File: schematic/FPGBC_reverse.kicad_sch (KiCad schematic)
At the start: 7 parts, among them IC1 CH32V203C8T6, J1 Conn_01x06_Pin, U1 GW2AR-LV18EQ144PC8_17, U2 24C04C, U3 W25Q128JVS, U4 EA3058QD, U5 TCD8002D

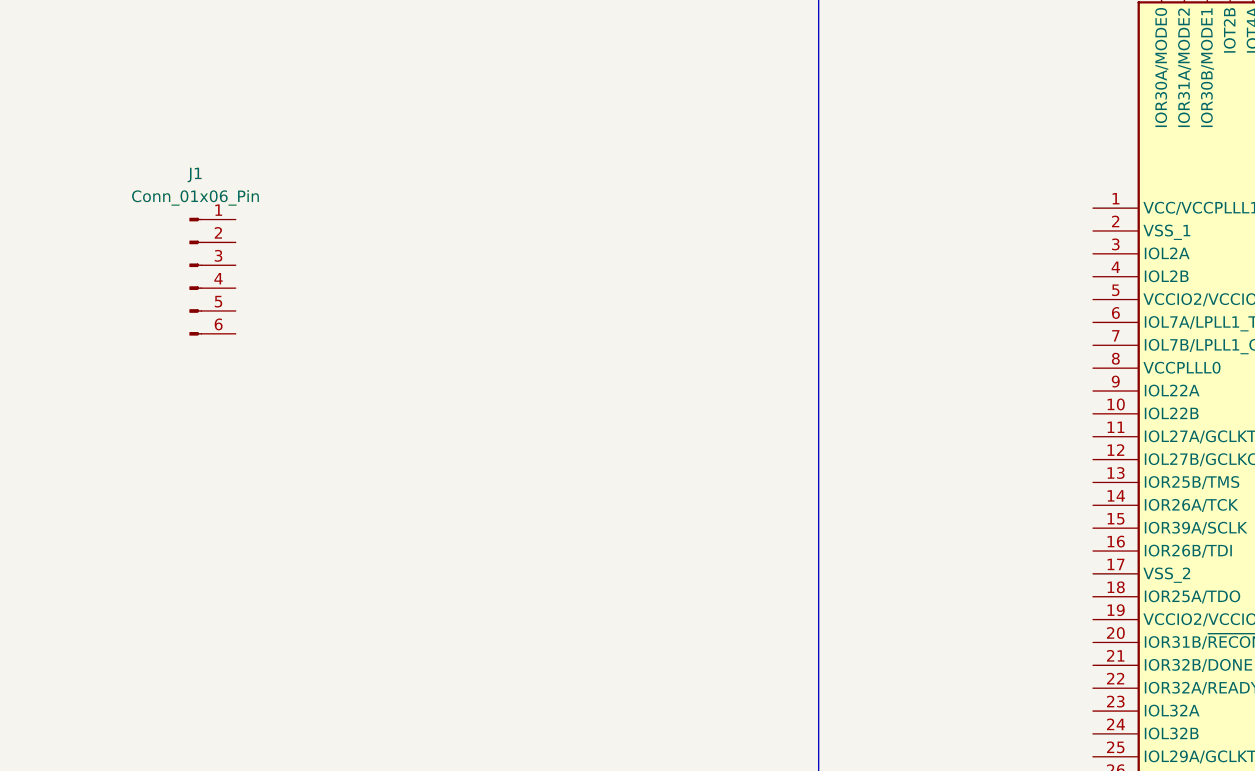
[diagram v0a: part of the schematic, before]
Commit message: más pines
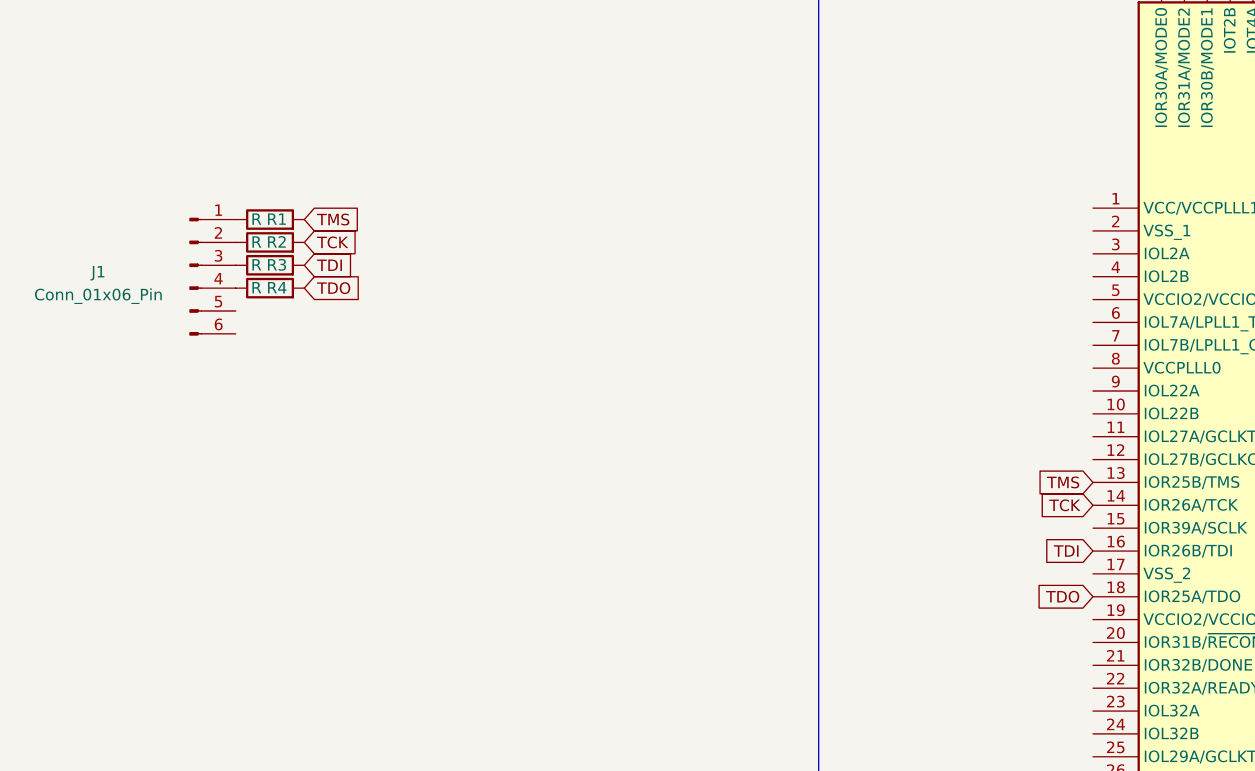
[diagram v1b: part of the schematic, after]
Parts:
- added R1, R2, R3, R4: R, Package_DIP:DIP-8_W7.62mm, symbol Device:R
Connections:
- net TMS: now reaches U1.13 (IOR25B/TMS)
- net TMS: now also R1.2
- net TCK: now reaches U1.14 (IOR26A/TCK)
- net TCK: now also R2.2
- net TDI: now reaches U1.16 (IOR26B/TDI)
- net TDI: now also R3.2
- net TDO: now reaches U1.18 (IOR25A/TDO)
- net TDO: now also R4.2
- net at J1.1 (Pin_1): now also R1.1
- net at J1.2 (Pin_2): now also R2.1
- net at J1.3 (Pin_3): now also R3.1
- net at J1.4 (Pin_4): now also R4.1

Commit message: Se agrega algunos IC al esquematico, se cambia el diagramad de bloques de conexiones, se añade preliminar de arquitectura en bloques
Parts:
- added J2: Conn_01x32_Socket, symbol Connector:Conn_01x32_Socket
- added U6: SN74LVC8T245, Package_SO:TSSOP-24_4.4x7.8mm_P0.65mm, symbol Logic_LevelTranslator:SN74LVC8T245
- added U7: TXB0104D, Package_SO:SOIC-14_3.9x8.7mm_P1.27mm, symbol Logic_LevelTranslator:TXB0104D
- U2: value 24C04C -> 24C04C EEPROM
- U3: value W25Q128JVS -> W25Q128JVS FLASH
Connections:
- net GBC_A0: now reaches U1.64 (IOB40A)
- net GBC_A0: now also J2.6 (Pin_6)
- net GBC_A1: now reaches U1.65 (IOB40B)
- net GBC_A1: now also J2.7 (Pin_7)
- net GBC_A2: now reaches U1.66 (IOB42A)
- net GBC_A2: now also J2.8 (Pin_8)
- net GBC_A3: now reaches U1.67 (IOB42B)
- net GBC_A3: now also J2.9 (Pin_9)
- net GBC_A4: now reaches U1.68 (IOB48A)
- net GBC_A4: now also J2.10 (Pin_10)
- net GBC_A5: now reaches U1.69 (IOB48B)
- net GBC_A5: now also J2.11 (Pin_11)
- net GBC_A6: now reaches U1.70 (IOB53A)
- net GBC_A6: now also J2.12 (Pin_12)
- net GBC_A7: now reaches U1.71 (IOB53B)
- net GBC_A7: now also J2.13 (Pin_13)
- net GBC_A8: now reaches U1.72 (IOB55B)
- net GBC_A8: now also J2.14 (Pin_14)
- net GBC_A9: now reaches U1.76 (IOR50B)
- net GBC_A9: now also J2.15 (Pin_15)
- net GBC_A10: now reaches U1.78 (IOR50A)
- net GBC_A10: now also J2.16 (Pin_16)
- net GBC_A11: now reaches U1.79 (IOR49B)
- net GBC_A11: now also J2.17 (Pin_17)
- net GBC_A12: now reaches U1.80 (IOR49A)
- net GBC_A12: now also J2.18 (Pin_18)
- net GBC_A13: now reaches U1.82 (IOR45A/RPLL2_T_IN)
- net GBC_A13: now also J2.19 (Pin_19)
- net GBC_A14: now reaches U1.83 (IOR42B)
- net GBC_A14: now also J2.20 (Pin_20)
- net GBC_A15: now reaches U1.84 (IOR42A)
- net GBC_A15: now also J2.21 (Pin_21)
- new net: J2.2 (Pin_2), U7.13 (B1)
- new net: U6.11 (GND), U6.12 (GND), U6.13 (GND)
- new net: U6.23 (V_{CCB}), U6.24 (V_{CCB})
- new net GBC#CS: J2.5 (Pin_5), U7.10 (B4)
- new net GBC#RD: J2.4 (Pin_4), U7.11 (B3)
- new net GBC#WR: J2.3 (Pin_3), U7.12 (B2)
- new net GBC_D0: J2.22 (Pin_22), U6.10 (A8), U6.14 (B8)
- new net GBC_D1: J2.23 (Pin_23), U6.15 (B7), U6.9 (A7)
- new net GBC_D2: J2.24 (Pin_24), U6.16 (B6), U6.8 (A6)
- new net GBC_D3: J2.25 (Pin_25), U6.17 (B5), U6.7 (A5)
- new net GBC_D4: J2.26 (Pin_26), U6.18 (B4), U6.6 (A4)
- new net GBC_D5: J2.27 (Pin_27), U6.19 (B3), U6.5 (A3)
- new net GBC_D6: J2.28 (Pin_28), U6.20 (B2), U6.4 (A2)
- new net GBC_D7: J2.29 (Pin_29), U6.21 (B1), U6.3 (A1)
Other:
- moved on the sheet: U2, U3, U4, U5
